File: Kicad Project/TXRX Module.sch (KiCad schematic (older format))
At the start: 16 parts, among them U10 GALI-2+, U11 BandpassFilter, U13 Antenna111, U14 Antenna111, U9 LEE-39+

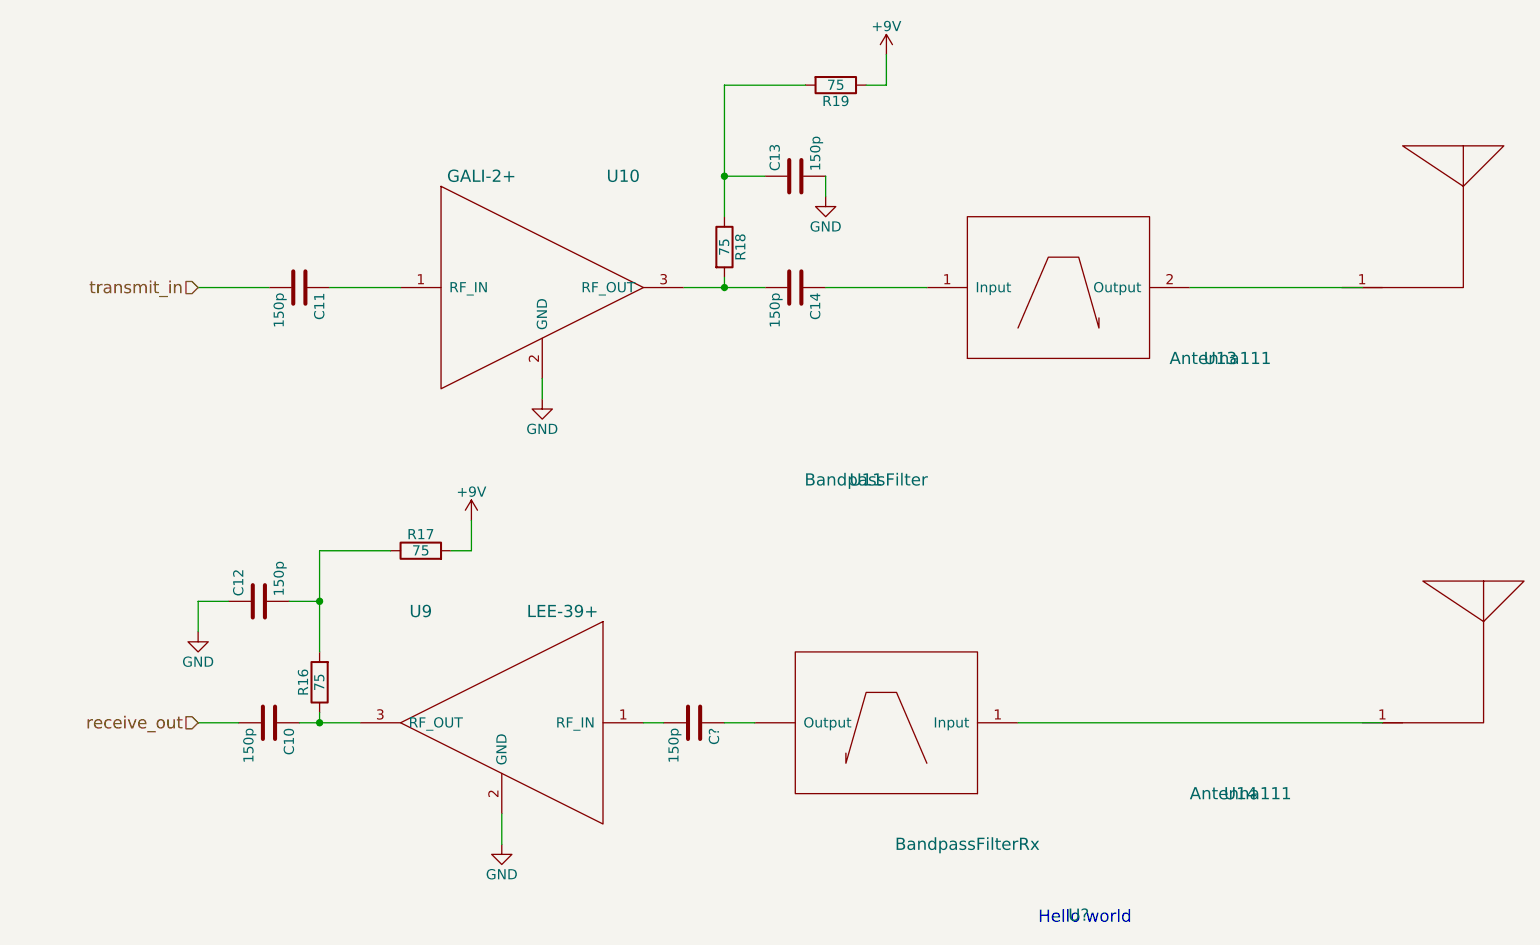
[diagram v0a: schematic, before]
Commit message: PCB LAYOUT update
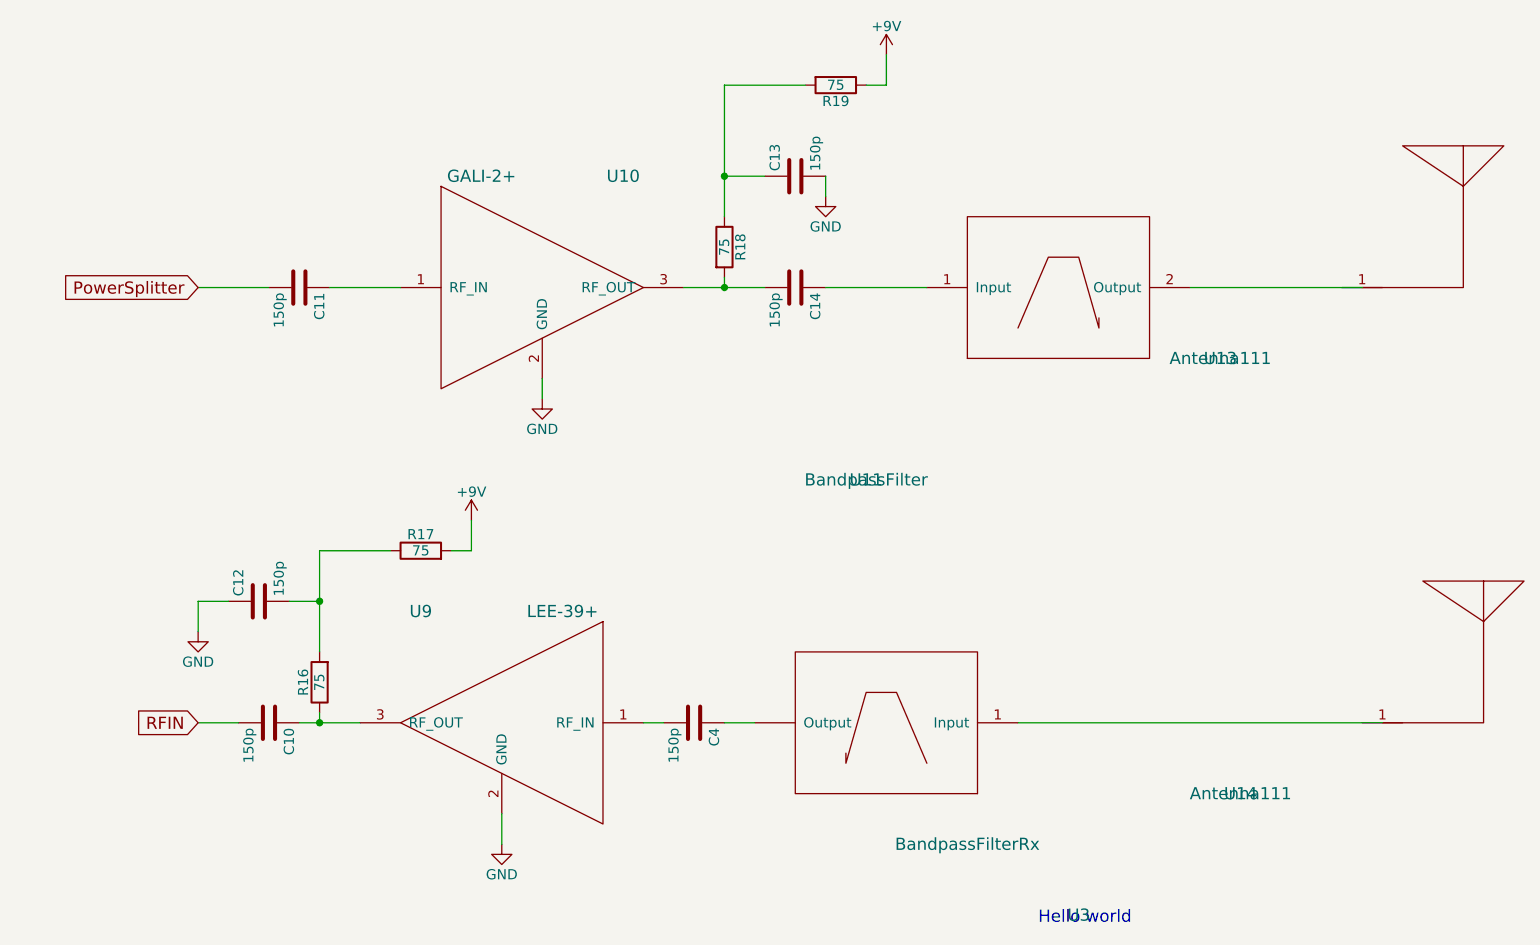
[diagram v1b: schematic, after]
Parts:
- gave numbers to parts that had none: 2
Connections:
- net labels added: PowerSplitter, RFIN
- net labels removed: receive_out, transmit_in
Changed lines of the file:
@@
 Text Notes 6500 5800 0    60   ~ 0
 Hello world
-Text HLabel 2350 2650 0    60   Input ~ 0
-transmit_in
-Text HLabel 2350 4800 0    60   Input ~ 0
-receive_out
 $Comp
 L C C11
@@
 $EndComp
 $Comp
-L GND #PWR015
+L GND #PWR011
 U 1 1 59FFE5A2
 P 2350 4350
-F 0 "#PWR015" H 2350 4100 50  0001 C CNN
+F 0 "#PWR011" H 2350 4100 50  0001 C CNN
 F 1 "GND" H 2350 4200 50  0000 C CNN
 F 2 "" H 2350 4350 50  0001 C CNN
@@
 $EndComp
 $Comp
-L GND #PWR016
+L GND #PWR012
 U 1 1 59FFE5D4
 P 3850 5400
-F 0 "#PWR016" H 3850 5150 50  0001 C CNN
+F 0 "#PWR012" H 3850 5150 50  0001 C CNN
 F 1 "GND" H 3850 5250 50  0000 C CNN
 F 2 "" H 3850 5400 50  0001 C CNN
@@
 $EndComp
 $Comp
-L GND #PWR017
+L GND #PWR013
 U 1 1 59FFE606
 P 4050 3200
-F 0 "#PWR017" H 4050 2950 50  0001 C CNN
+F 0 "#PWR013" H 4050 2950 50  0001 C CNN
 F 1 "GND" H 4050 3050 50  0000 C CNN
 F 2 "" H 4050 3200 50  0001 C CNN
@@
 $EndComp
 $Comp
-L GND #PWR018
+L GND #PWR014
 U 1 1 59FFE638
 P 5450 2200
-F 0 "#PWR018" H 5450 1950 50  0001 C CNN
+F 0 "#PWR014" H 5450 1950 50  0001 C CNN
 F 1 "GND" H 5450 2050 50  0000 C CNN
 F 2 "" H 5450 2200 50  0001 C CNN
@@
 	2350 4800 2550 4800
 $Comp
-L +9V #PWR?
+L +9V #PWR015
 U 1 1 5A01141C
 P 5750 1500
-F 0 "#PWR?" H 5750 1350 50  0001 C CNN
+F 0 "#PWR015" H 5750 1350 50  0001 C CNN
 F 1 "+9V" H 5750 1640 50  0000 C CNN
 F 2 "" H 5750 1500 50  0001 C CNN
@@
 $EndComp
 $Comp
-L +9V #PWR?
+L +9V #PWR016
 U 1 1 5A0114D0
 P 3700 3800
-F 0 "#PWR?" H 3700 3650 50  0001 C CNN
+F 0 "#PWR016" H 3700 3650 50  0001 C CNN
 F 1 "+9V" H 3700 3940 50  0000 C CNN
 F 2 "" H 3700 3800 50  0001 C CNN
@@
 	5750 1650 5750 1500
 $Comp
-L BandpassFilterRx U?
+L BandpassFilterRx U3
 U 1 1 5A012078
 P 6700 5750
-F 0 "U?" H 6700 5750 60  0000 C CNN
+F 0 "U3" H 6700 5750 60  0000 C CNN
 F 1 "BandpassFilterRx" H 7250 6100 60  0000 C CNN
 F 2 "" H 6700 5750 60  0001 C CNN
@@
 $EndComp
 $Comp
-L C C?
+L C C4
 U 1 1 5A012959
 P 4800 4800
-F 0 "C?" H 4825 4900 50  0000 L CNN
+F 0 "C4" H 4825 4900 50  0000 L CNN
 F 1 "150p" H 4825 4700 50  0000 L CNN
 F 2 "" H 4838 4650 50  0001 C CNN
@@
 Wire Wire Line
 	4650 4800 4550 4800
+Text GLabel 2350 2650 0    60   Input ~ 0
+PowerSplitter
+Text GLabel 2350 4800 0    60   Input ~ 0
+RFIN
 $EndSCHEMATC
